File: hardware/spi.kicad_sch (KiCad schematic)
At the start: 7 parts, among them J2 DeadOn RTC, J3 Micro_SD_Card

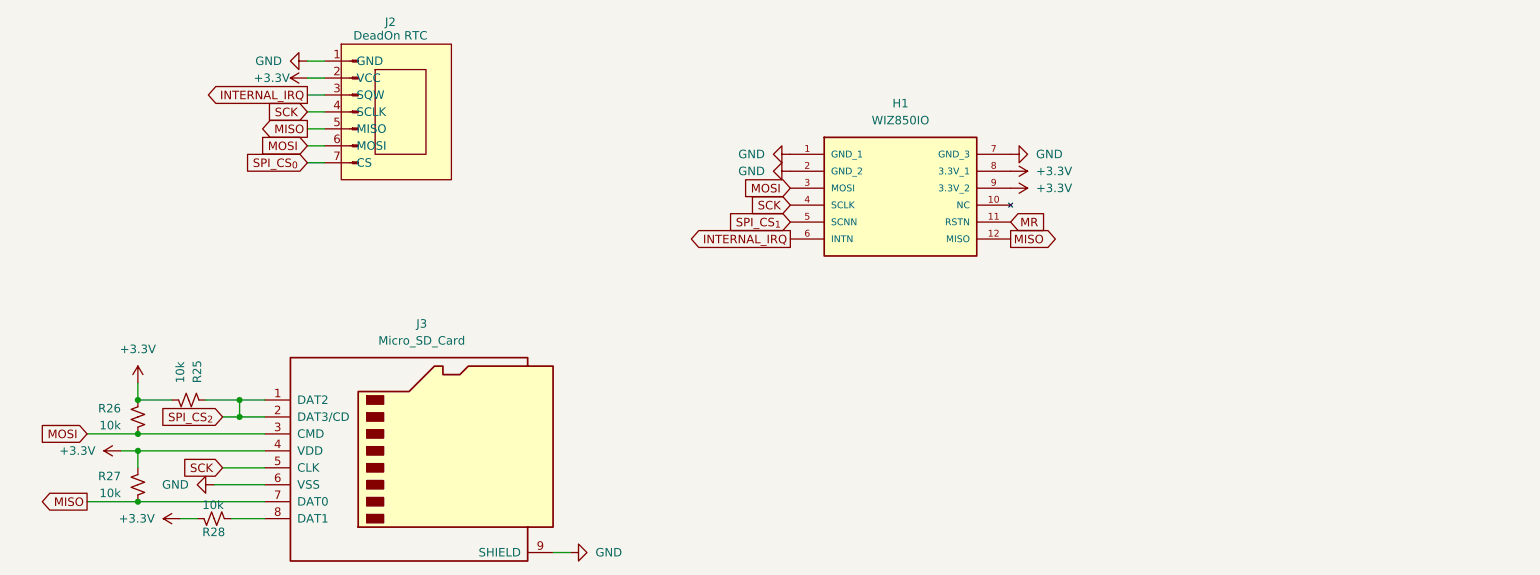
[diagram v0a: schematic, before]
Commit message: Fixes and addres fix adding VDA AND VPA
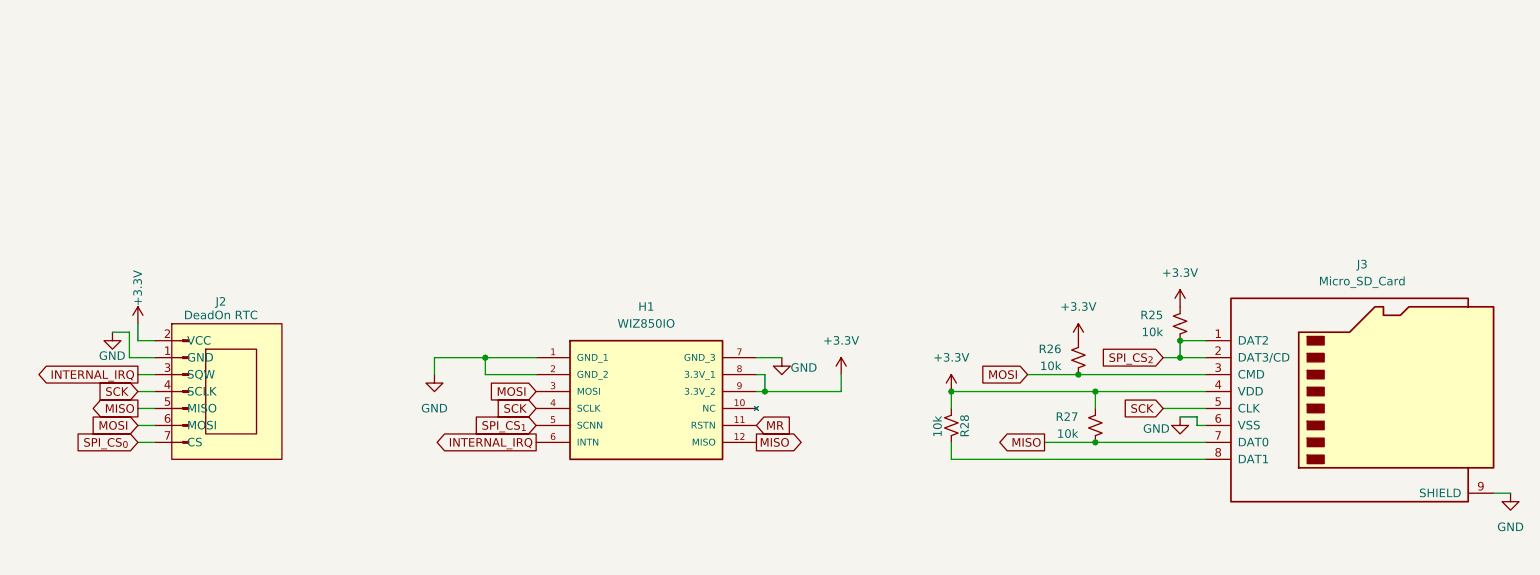
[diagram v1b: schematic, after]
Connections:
- net +3.3V: now also R25.1, R28.1; no longer R25.2, R28.2
- net SPI_CS_{2}: now also R25.2; no longer R25.1
- net at J3.8 (DAT1): now also R28.2; no longer R28.1
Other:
- moved on the sheet: H1, J2, J3, R25, R26, R27, R28
